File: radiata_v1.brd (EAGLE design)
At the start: 80 x 80 mm, 93 parts, among them IC2 MEGA48/88/168-AU, Q1 FA-20H

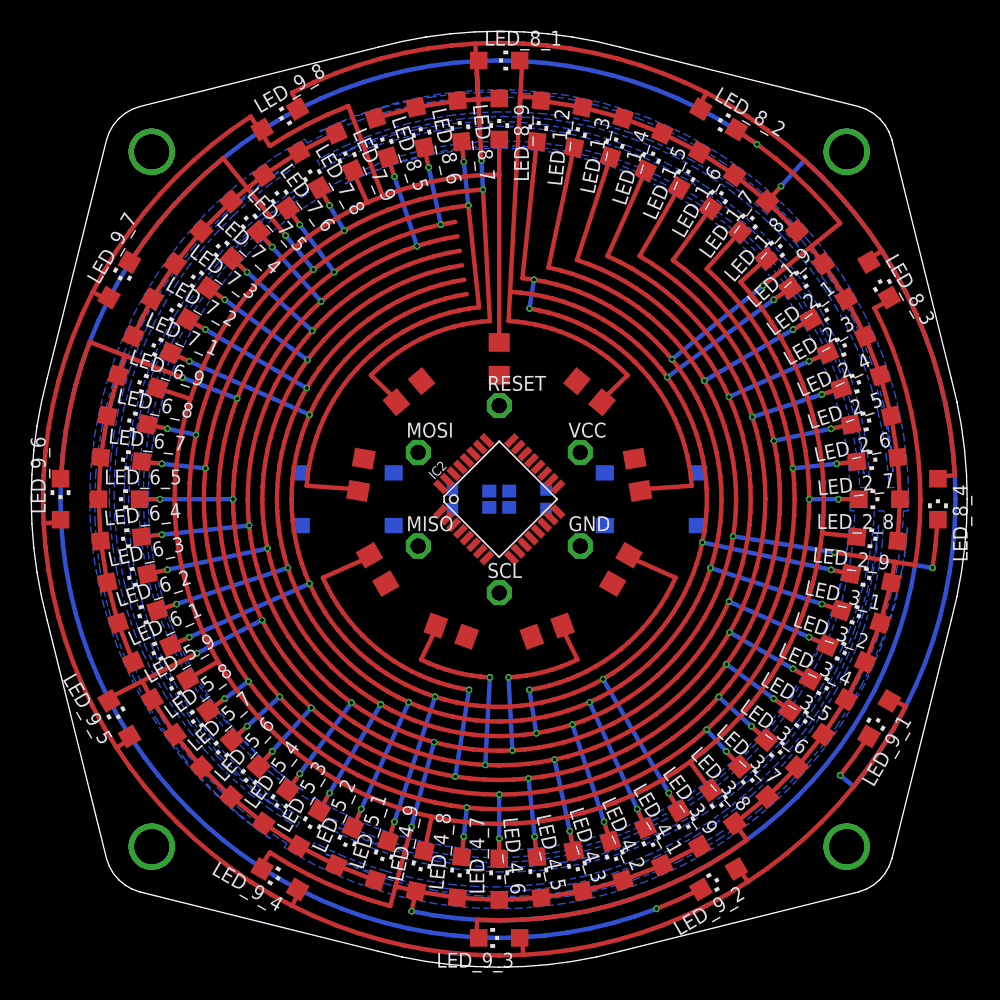
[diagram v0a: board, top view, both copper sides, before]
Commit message: lots of progress, driving towards a scroll wheel that passes DRC
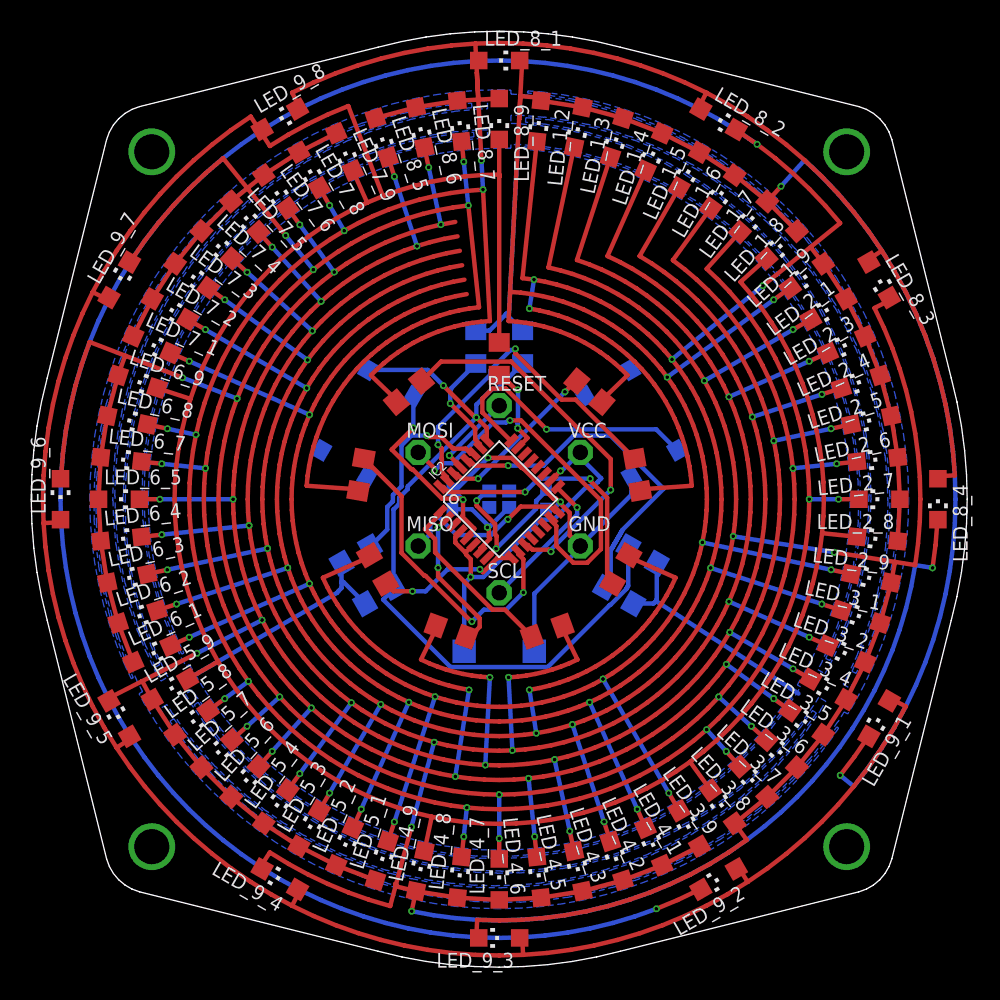
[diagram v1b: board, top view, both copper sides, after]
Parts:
- added GND2, V+: PTR1TP20SQ, testpad:TP20SQ
- added RR1, RR2, RR3, RS1, RS2, RS3: (no value), SparkFun:1206
- moved DOWNSW 6.73 mm to (28.7, 46.5), turned to 120 degrees
- moved UPSW 6.73 mm to (51.3, 46.5), turned to 240 degrees
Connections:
- new net ROTOR1: RR1.1, RS1.2
- new net ROTOR2: RR2.1, RS2.2
- new net ROTOR3: RR3.1, RS3.2
- net GND: now also GND2.TP
- net PC2: now also RS1.1, RS2.1, RS3.1
- net PC3: now also RR1.2
- net PC4: now also RR2.2
- net PC5: now also RR3.2
- net VCC: now also V+.TP
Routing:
- net PC2: track 0.00 -> 68.3 mm, vias 0 -> 2
- net GND: track 0.00 -> 56.7 mm, vias 0 -> 4
- net VCC: track 0.00 -> 33.3 mm, vias 0 -> 2
- net PD7: track 0.00 -> 32.9 mm, vias 0 -> 2
- net N$8: track 0.00 -> 32.6 mm, vias 0 -> 2
- net PC5: track 0.00 -> 30.4 mm, vias 0 -> 1
- net PD1: track 0.00 -> 28.8 mm, vias 0 -> 2
- net PD6: track 0.00 -> 27.0 mm, vias 0 -> 2
- net PC1: track 0.00 -> 23.9 mm, vias 0 -> 1
- net PD2: track 0.00 -> 23.2 mm, vias 0 -> 2
- net ROTOR1: track 0.00 -> 20.0 mm
- net ROTOR2: track 0.00 -> 20.0 mm
- net ROTOR3: track 0.00 -> 19.8 mm
- net PC4: track 0.00 -> 16.9 mm, vias 0 -> 1
- net PD3: track 0.00 -> 15.7 mm
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- added copper zone on layer 16, net ROTOR1
- added copper zone on layer 16, net ROTOR2
- added copper zone on layer 16, net ROTOR3
- removed copper zone on layer 16, net N$10
- removed copper zone on layer 16, net N$11
- removed copper zone on layer 16, net N$9
